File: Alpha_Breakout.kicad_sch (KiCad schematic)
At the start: 0 parts

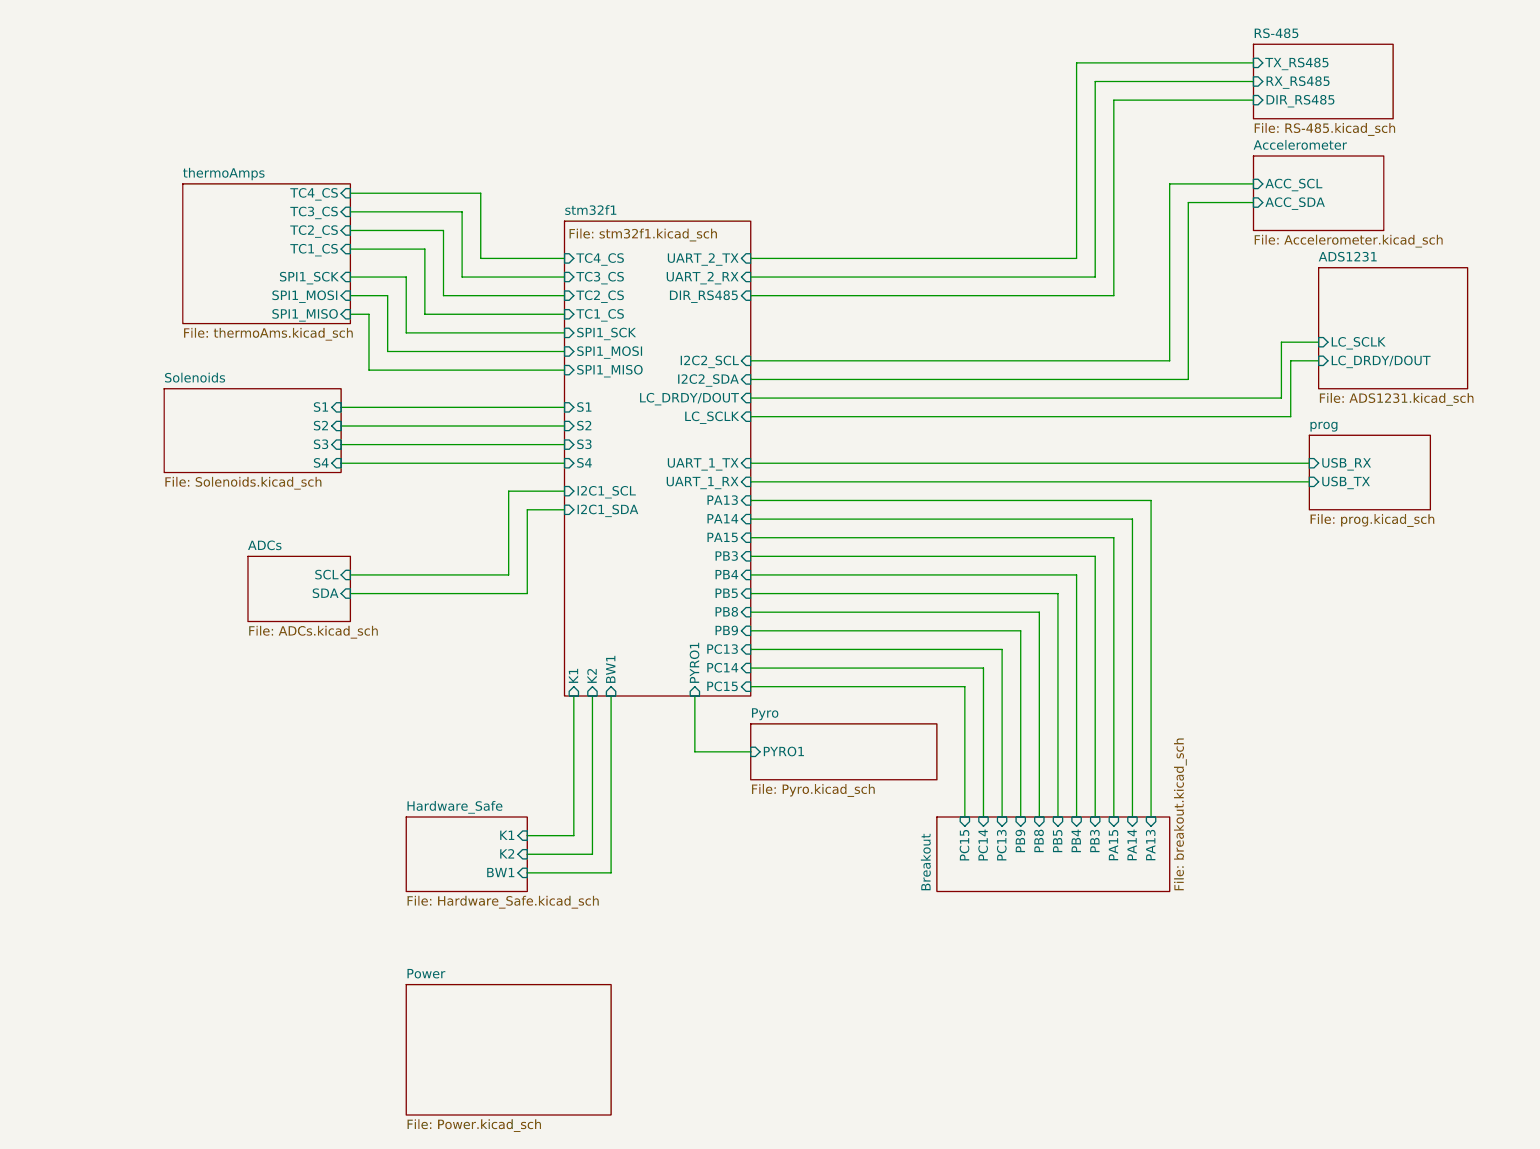
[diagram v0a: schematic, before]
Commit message: lots🅿️
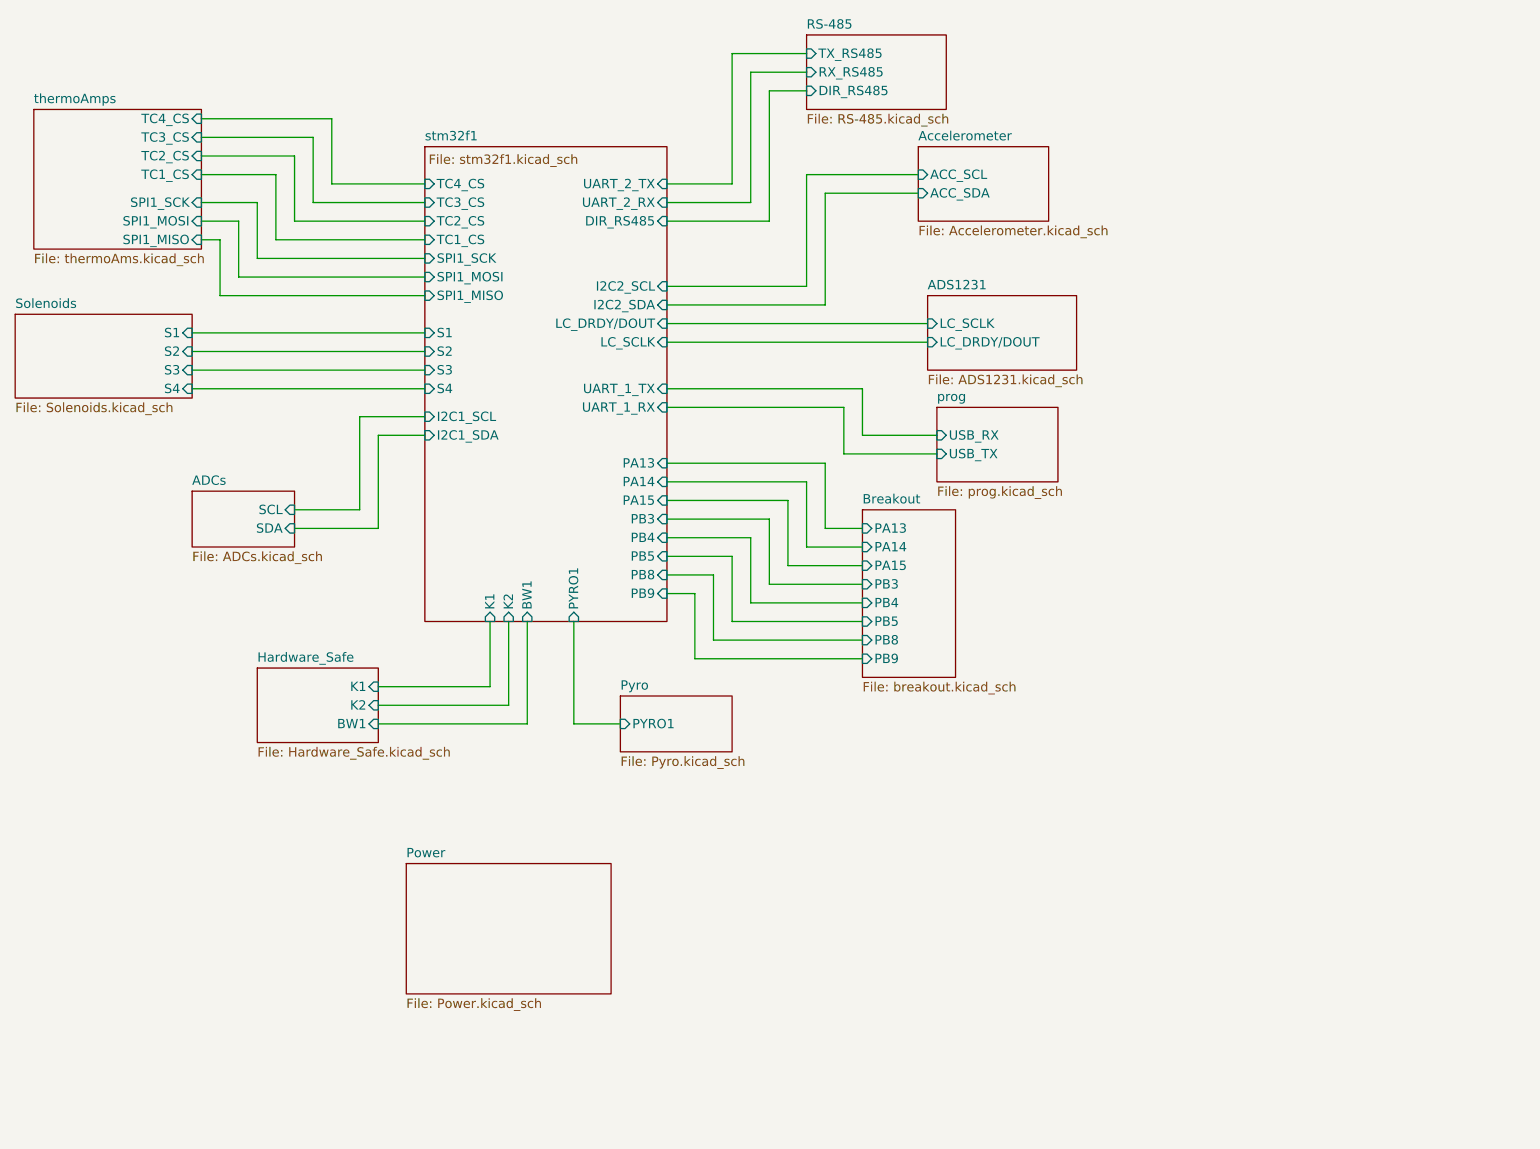
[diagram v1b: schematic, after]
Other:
- sheet Breakout ports: added none; removed PC13, PC14, PC15
- sheet stm32f1 ports: added none; removed PC13, PC14, PC15
